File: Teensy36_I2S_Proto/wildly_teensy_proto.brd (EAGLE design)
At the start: 96.2 x 82.5 mm, 34 parts, among them SW2 Push_Button

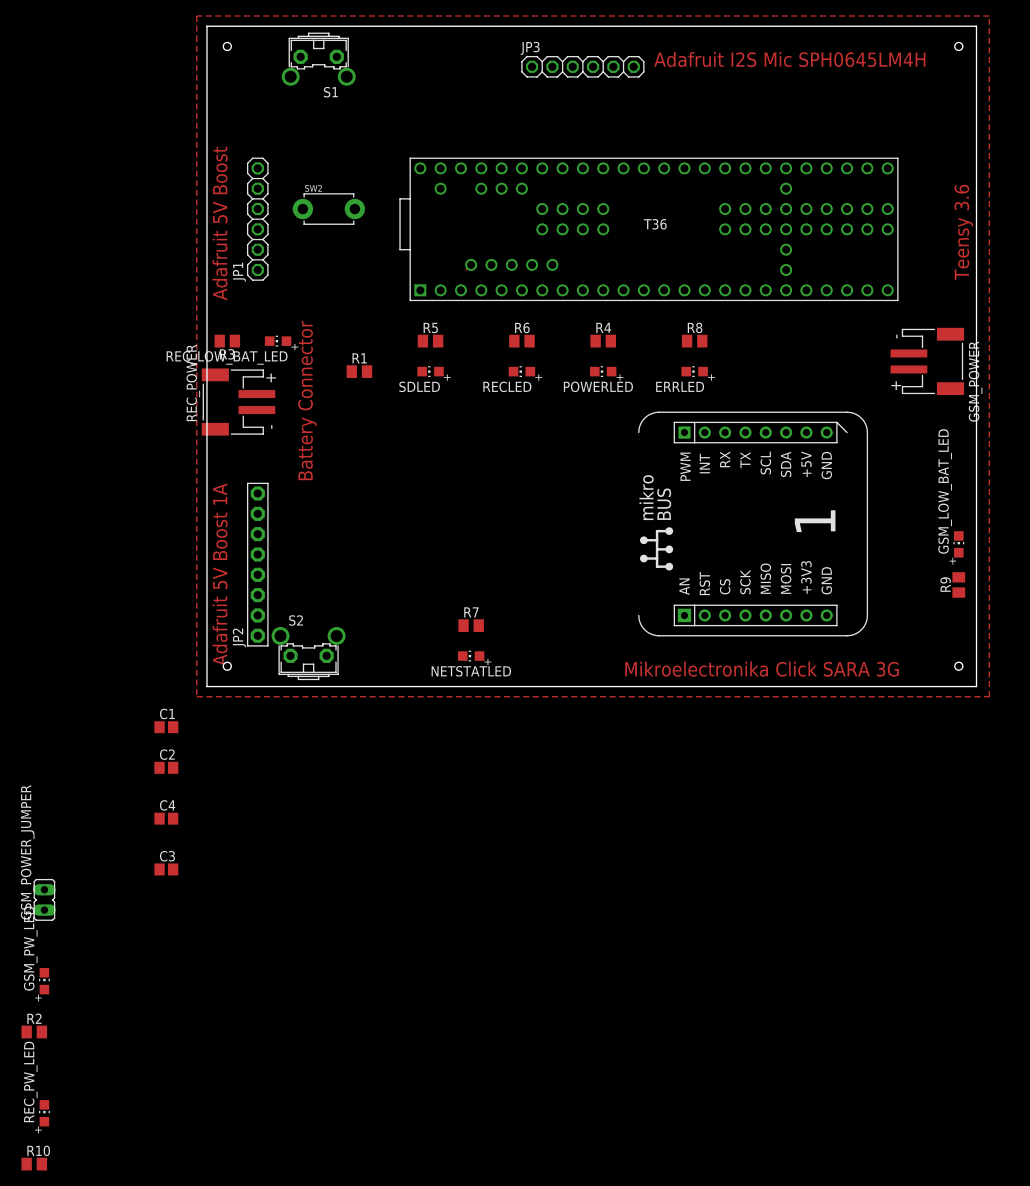
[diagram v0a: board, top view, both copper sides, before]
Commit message: Remove LEDs for Power Enables, Remove LEDs for Low Bat indicators, Add NPN Transistors as LED drivers - TBD: Calculate R values, Remove Power LED and change pinout to power control for resetting system power- TBD: add connection, Provide 3.3V to GSM modem
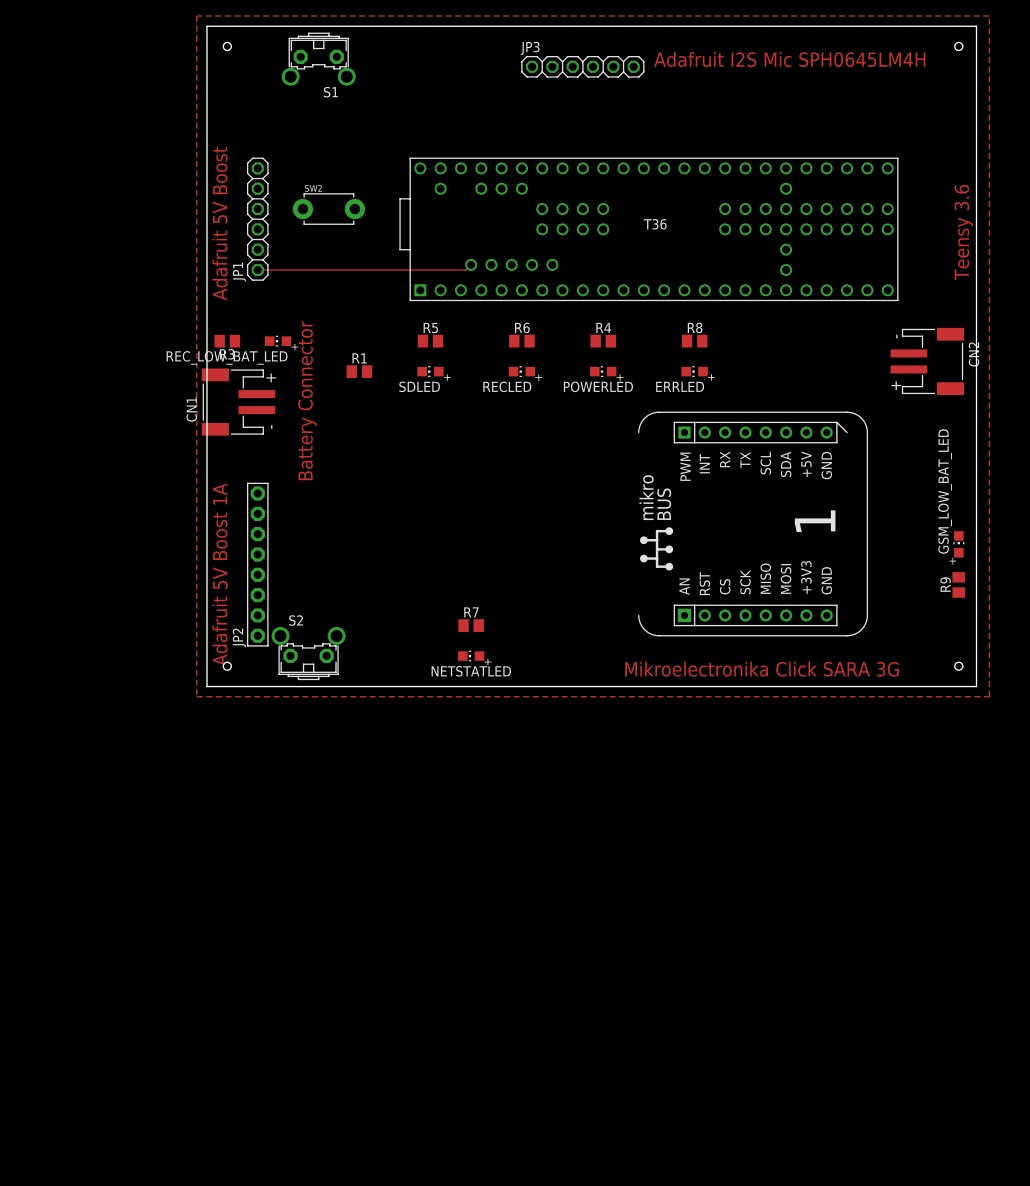
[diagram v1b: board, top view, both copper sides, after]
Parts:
- removed C1, C3: 10uF, adafruit:C0805
- removed C2, C4: 100nF, adafruit:C0805
- removed GSM_POWER_JUMPER: (no value), jumper:JP1
- removed GSM_PW_LED, REC_PW_LED: (no value), adafruit:CHIP-LED0805
- removed R10, R2: 1KR, adafruit:M0805
- R3, R4, R5, R6, R7, R8, R9: value 1KR -> 330R
- renumbered GSM_POWER to CN2, MIKROELECTRONIKA_SARA_CLICK to CON1, REC_POWER to CN1
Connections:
- net GSM_BAT renamed N$24
- net GSM_LB renamed N$20
- net MIC_3V renamed 3V
- net MIC_BCLK renamed BCLK
- net MIC_DOUT renamed DOUT
- net MIC_LRCLK renamed LRCLK
- net NETSTATLED renamed N$21
- net REC_BAT renamed N$3
- net REC_LB renamed N$10
- removed net ERRLED: R8.1, U$1.39
- removed net GSM_5V: C3.1, C4.1, CON1.P$10, GSM_POWER_JUMPER.1, JP2.1
- removed net GSM_5V_EN: JP2.5, R10.1
- removed net GSM_BAT_RETURN: CN2.2, JP2.4
- removed net N$10 (its old number): R2.1, REC_PW_LED.A
- removed net N$3 (its old number): POWERLED.A, R4.2
- removed net N$6: JP2.6
- removed net POWERLED: R4.1, U$1.35
- removed net RECLED: R6.1, U$1.36
- removed net REC_5V: C1.1, C2.1, GSM_POWER_JUMPER.2, JP1.1, U$1.5V
- removed net REC_5V_EN: JP1.4, REC_PW_LED.C, S1.2
- removed net REC_BAT_RETURN: CN1.2, JP1.5
- removed net SDLED: R5.1, U$1.37
- new net N$13: R6.2, U$1.36
- new net N$14: R8.1, U$1.37
- new net N$15: POWERLED.A, R4.1
- new net N$17: CN1.2
- new net N$18: JP1.5
- new net N$19: JP2.5, S2.2
- new net N$2: JP1.1, U$1.5V
- new net N$25: CON1.P$10, JP2.1
- net GND: now also CN2.2, JP2.4, S1.2, S2.1; no longer C1.2, C2.2, C3.2, C4.2, S1.1, S2.2
- net N$12: now also R5.1, U$1.39; no longer R2.2
- net N$4: now also JP1.4, S1.1; no longer GSM_PW_LED.A, R10.2
- net N$5: now also R4.2, U$1.35; no longer GSM_PW_LED.C, S2.1
- net N$9: now also R6.1; no longer R6.2
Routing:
- net N$2: track 0.00 -> 26.9 mm
- net REC_5V: track 0.90 -> 0.00 mm
